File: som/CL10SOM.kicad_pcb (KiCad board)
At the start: 4 copper layers, 34 x 32 mm, 56 parts, among them IC1 10CL025YU256C8G, U1 MT46H32M16LFBF-5 IT:C, U2 MX25L12833FM2, U3 SC189ZSKTRT, U4 SC189CSKTRT, U6 AT93C46DN-SH-T, U7 SG3225CAN 50.0000M-TJGA6, X1 DF40C-120DS-0.4V51

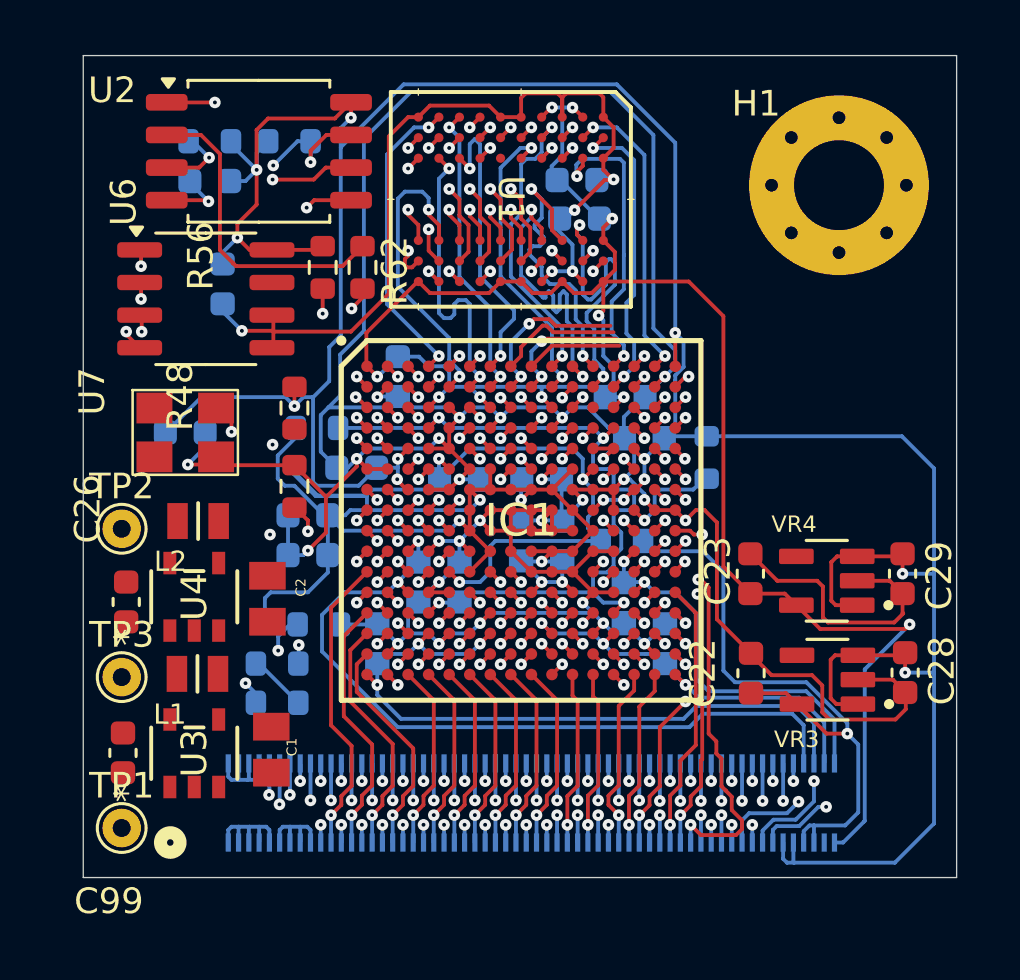
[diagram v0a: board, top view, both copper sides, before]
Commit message: All routed, no errors
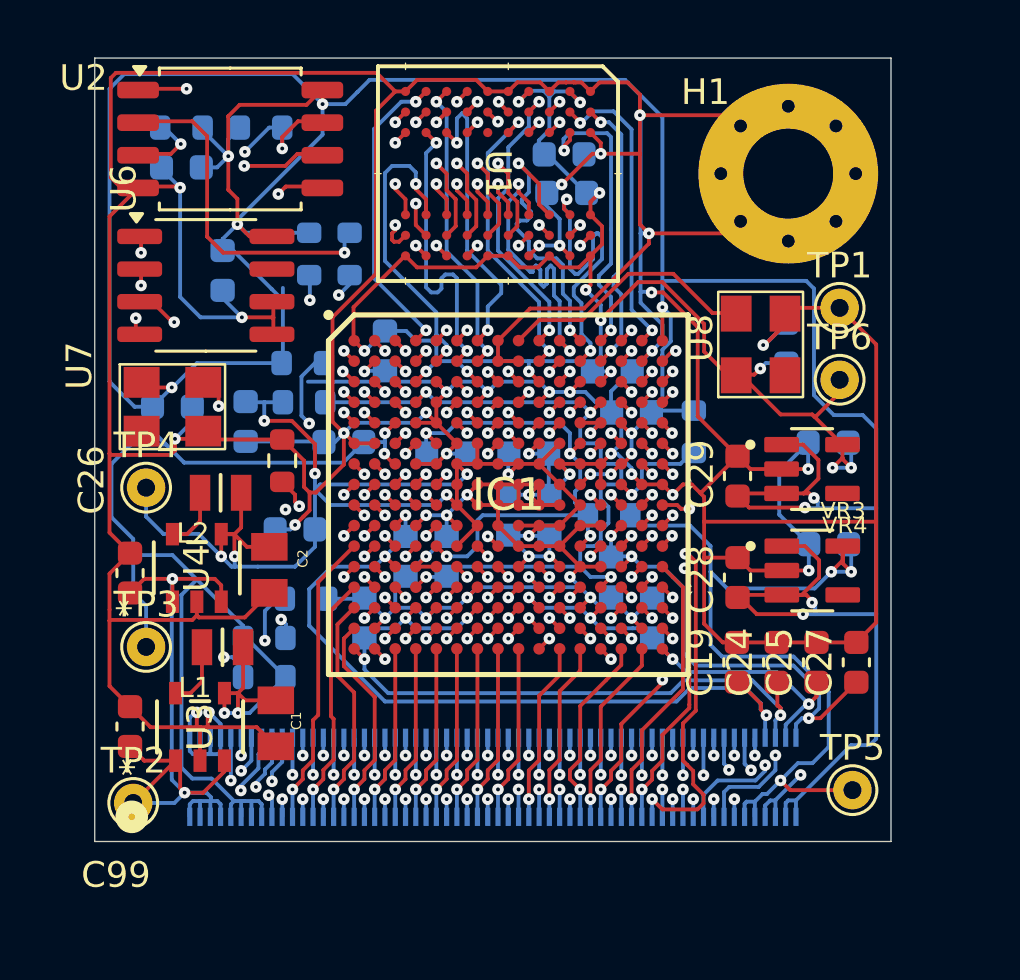
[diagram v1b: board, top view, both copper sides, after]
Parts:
- added C10: 100nF, Capacitor_SMD:C_0603_1608Metric, B.Cu at (110.7, 55.6)
- added C19: 100nF, Capacitor_SMD:C_0603_1608Metric, F.Cu at (108.8, 68.0)
- added C24: 100nF, Capacitor_SMD:C_0603_1608Metric, F.Cu at (110.3, 68.0)
- added C25: 100nF, Capacitor_SMD:C_0603_1608Metric, F.Cu at (111.8, 68.0)
- added C27: 100nF, Capacitor_SMD:C_0603_1608Metric, F.Cu at (113.4, 68.0)
- added TP4: TestPoint, TestPoint:TestPoint_THTPad_D1.5mm_Drill0.7mm, F.Cu at (85.8, 61.2)
- added TP5: TestPoint, TestPoint:TestPoint_THTPad_D1.5mm_Drill0.7mm, F.Cu at (113.2, 73.0)
- added TP6: TestPoint, TestPoint:TestPoint_THTPad_D1.5mm_Drill0.7mm, F.Cu at (112.8, 57.0)
- added U8: SG3225CAN 50.0000M-TJGA6, Library:SG3225CAN, F.Cu at (109.7, 55.6)
- C22, C23, R48, R56, R62: moved to B.Cu
- moved TP1 34.5 mm to (112.8, 54.2)
- moved TP2 10.7 mm to (85.2, 73.5)
- moved C28 7.50 mm to (108.8, 64.7), turned to -90 degrees
- moved C29 7.46 mm to (108.8, 60.8), turned to -90 degrees
- moved C23 5.93 mm to (112.3, 59.5), turned to 0 degrees
- moved C22 5.87 mm to (112.3, 63.4), turned to 0 degrees
- moved VR4 4.39 mm to (111.7, 60.5), turned to 0 degrees
- moved C45 4.38 mm to (89.6, 58.6), turned to -90 degrees
- moved VR3 4.29 mm to (111.7, 64.5), turned to 0 degrees
- moved H1 2.03 mm to (110.8, 49.0)
- moved X1 1.80 mm to (99.2, 72.5)
- moved R48 1.78 mm to (91.8, 56.4), turned to 0 degrees
- moved TP3 1.51 mm to (85.8, 67.4)
- moved L1 1.42 mm to (88.7, 67.4)
- moved L2 1.41 mm to (88.7, 61.4)
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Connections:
- IC1 pad A8: /B8-CLK10 -> GND
- IC1 pad A9: /B7-CLK8 -> /CLCOPT
- IC1 pad B8: /B8-CLK11 -> GND
- IC1 pad B9: /B7-CLK9 -> GND
- IC1 pad N8: /B3-IO15 -> /B3-IO16
- IC1 pad P8: /B3-IO16 -> /B3-IO17
- X1 pad 109: +3V3 -> +2V5
- X1 pad 111: +3V3 -> +2V5
- X1 pad 113: +2V5 -> +1V8
- X1 pad 115: +2V5 -> +1V8
- X1 pad 117: +1V8 -> +3V3
- X1 pad 119: +1V8 -> +3V3
- X1 pad 17: +3V3 -> +2V5
- X1 pad 54: /B3-IO15 -> /B3-IO16
- X1 pad 56: /B3-IO16 -> /B3-IO17
- X1 pad 9: +5V -> +3V3
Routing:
- net GND: track 219.2 -> 327.3 mm, vias 34 -> 43
- net +3V3: track 131.8 -> 203.6 mm, vias 13 -> 17
- net +2V5: track 24.7 -> 54.3 mm, vias 1 -> 4
- net +5V: track 4.54 -> 28.8 mm, vias 0 -> 2
- net +1V2: track 44.0 -> 58.0 mm, vias 6 -> 10
- net /CLCOPT: track 0.00 -> 10.2 mm
- net PLLA: track 29.7 -> 20.2 mm
- net /B3-IO15: track 18.1 -> 9.20 mm, vias 4 -> 2
- net /B3-IO17: track 0.00 -> 7.39 mm, vias 0 -> 2
- net /B8-CLK11: track 6.54 -> 0.00 mm, vias 2 -> 0
- net +1V8: track 75.8 -> 81.9 mm, vias 10 -> 14
- net /B7-CLK9: track 5.22 -> 0.00 mm, vias 2 -> 0
- net /B8-CLK10: track 4.96 -> 0.00 mm
- net /TDO: track 14.1 -> 17.9 mm
- net /B7-CLK8: track 3.76 -> 0.00 mm
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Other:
- board size 34 x 32 mm -> 31 x 30.5 mm
